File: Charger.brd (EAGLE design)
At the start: 160 x 100 mm, 14 parts, among them Q1 SPP80P06P

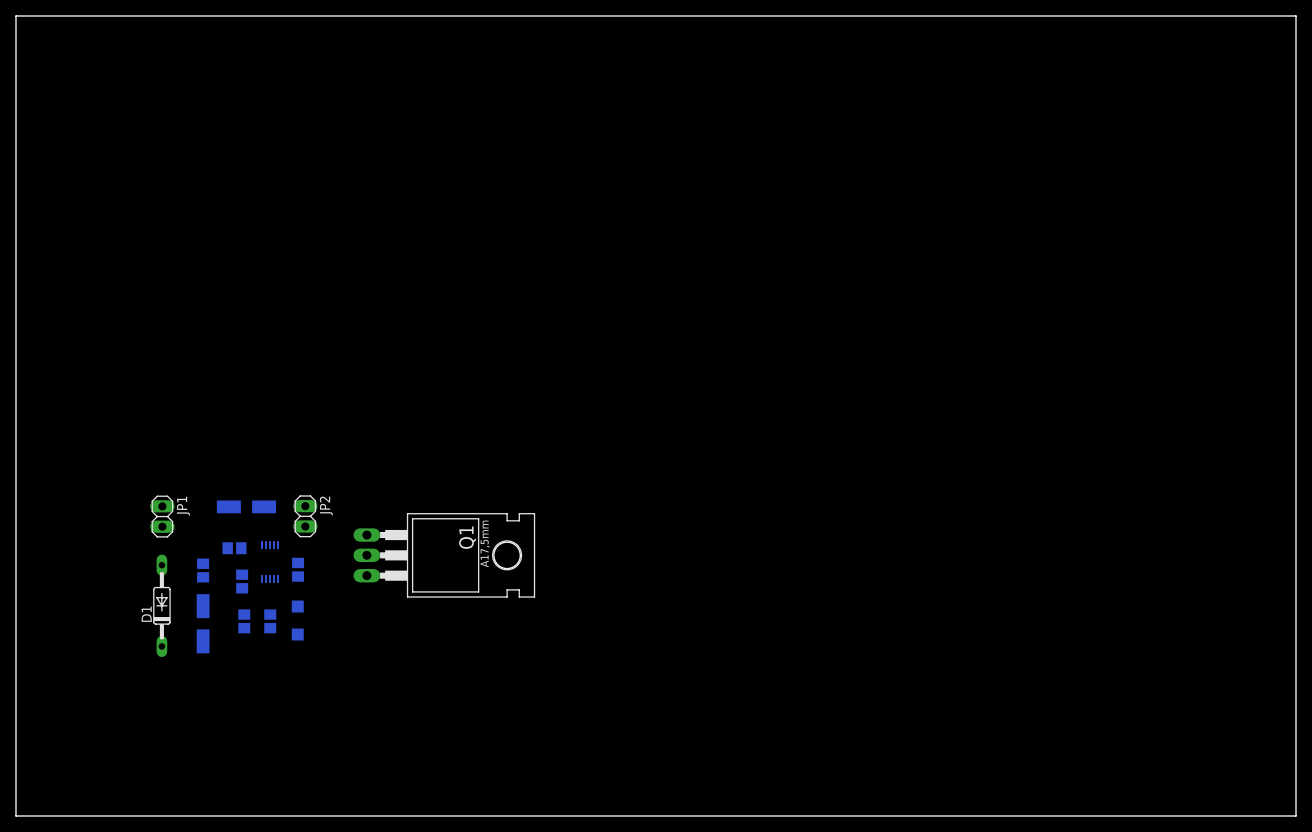
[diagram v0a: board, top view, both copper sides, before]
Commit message: Finished BRD
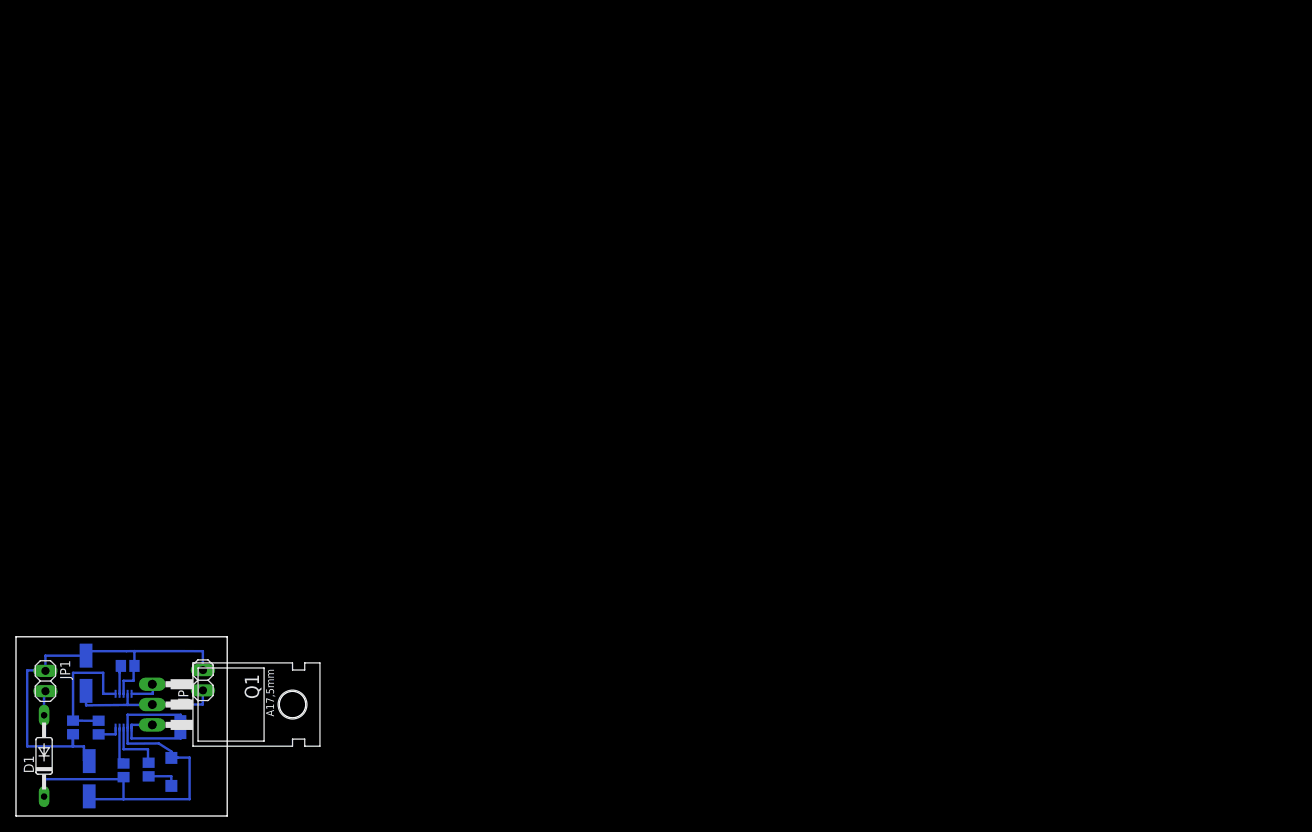
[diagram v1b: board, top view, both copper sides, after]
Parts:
- moved Q1 32.7 mm to (23.4, 13.9)
- moved R4 30.1 mm to (7.13, 11.1), turned to 90 degrees
- moved C1 28.9 mm to (8.76, 17.8), turned to 270 degrees
- moved U$1 26.1 mm to (13.4, 13.2)
- moved R3 25.6 mm to (10.3, 11.1)
- moved JP1 25.2 mm to (3.68, 16.9)
- moved LED1 24.6 mm to (19.4, 5.51)
- moved R1 24.6 mm to (20.5, 11.1), turned to 270 degrees
- moved JP2 24.2 mm to (23.4, 17.0), turned to 90 degrees
- moved C3 24.0 mm to (9.15, 4.66)
- moved R2 24.0 mm to (13.4, 5.71)
- moved R5 24.0 mm to (16.6, 5.81)
- moved D1 23.9 mm to (3.51, 7.51)
- moved C2 15.2 mm to (14.0, 18.8), turned to 180 degrees
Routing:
- net GND: track 0.00 -> 55.7 mm
- net N$1: track 0.00 -> 53.2 mm
- net N$7: track 0.00 -> 19.8 mm
- net N$12: track 0.00 -> 17.5 mm
- net N$2: track 0.00 -> 11.4 mm
- net N$6: track 0.00 -> 7.52 mm
- net N$3: track 0.00 -> 4.99 mm
- net N$4: track 0.00 -> 4.04 mm
- net N$5: track 0.00 -> 3.94 mm
- net N$8: track 0.00 -> 3.56 mm
- net N$10: track 0.00 -> 3.18 mm
- net N$11: track 0.00 -> 2.96 mm
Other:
- board size 160 x 100 mm -> 26.4 x 22.4 mm
